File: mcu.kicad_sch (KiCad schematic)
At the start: 15 parts, among them SW1 RST, SW2 BOOT, U1 ESP32-S3-WROOM-1

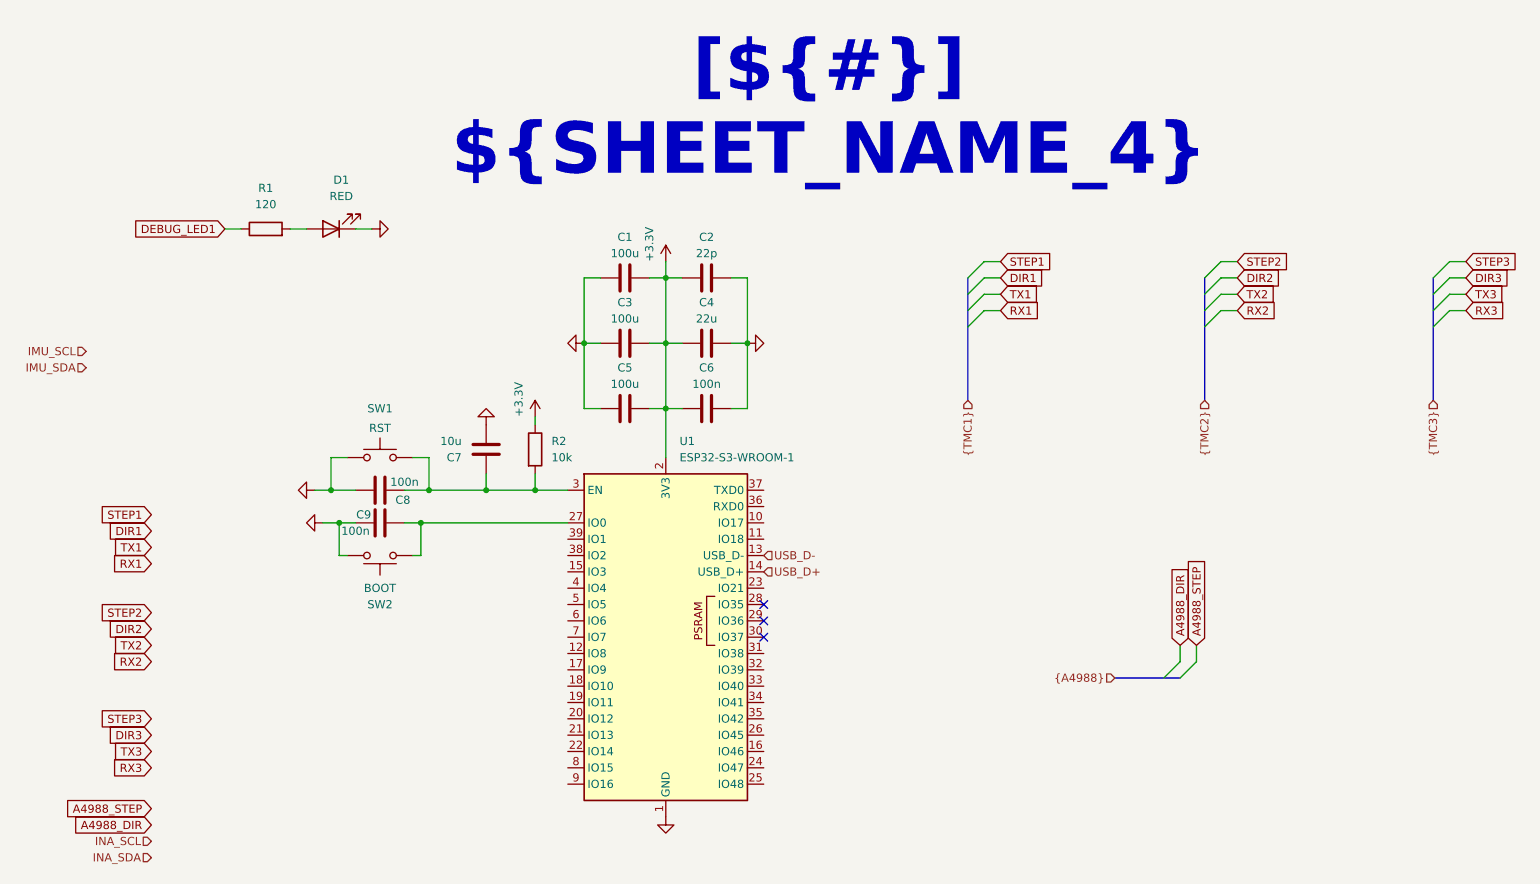
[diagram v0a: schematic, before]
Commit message: Finished design
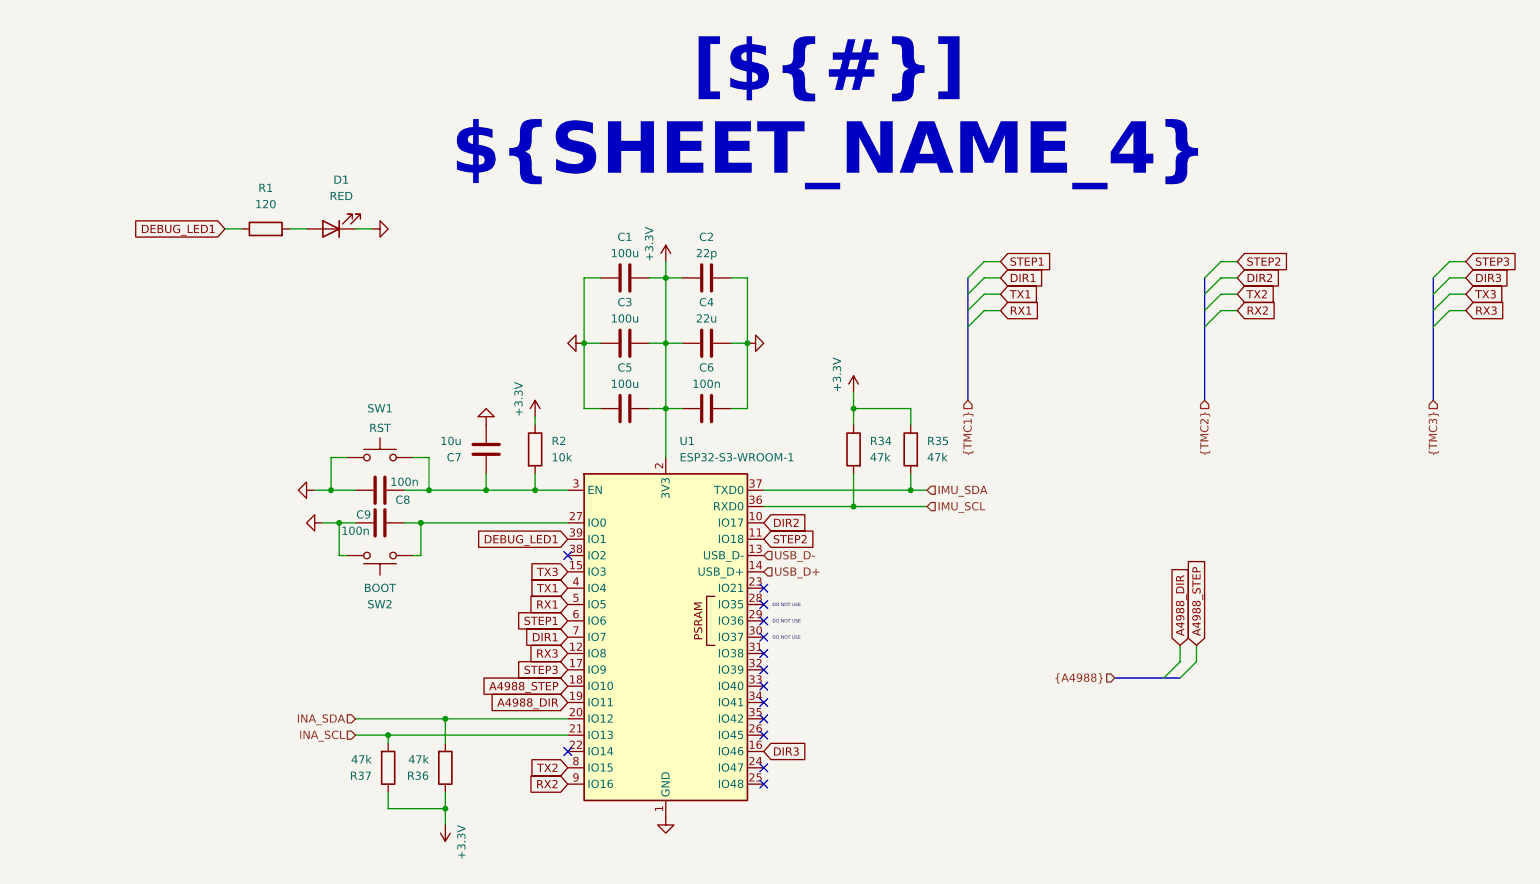
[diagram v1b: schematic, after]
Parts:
- added R34, R35, R36, R37: 47k, Resistor_SMD:R_0603_1608Metric_Pad0.98x0.95mm_HandSolder, symbol Device:R
- C1, C2, C3, C4, C5, C6, C7, C8, C9: footprint (none) -> Capacitor_SMD:C_0603_1608Metric_Pad1.08x0.95mm_HandSolder
- D1: footprint (none) -> LED_SMD:LED_0603_1608Metric_Pad1.05x0.95mm_HandSolder
- R1, R2: footprint (none) -> Resistor_SMD:R_0603_1608Metric_Pad0.98x0.95mm_HandSolder
- U1: footprint (none) -> Project_Components:ESP32-S3-WROOM-1_novias
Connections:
- net +3.3V: now also R34.1, R35.1, R36.1, R37.1
- net A4988_DIR: now also U1.19 (IO11)
- net A4988_STEP: now also U1.18 (IO10)
- net DEBUG_LED1: now also U1.39 (IO1)
- net DIR1: now also U1.7 (IO7)
- net DIR2: now also U1.10 (IO17)
- net DIR3: now also U1.16 (IO46)
- net IMU_SCL: now also U1.36 (RXD0), R34.2
- net IMU_SDA: now also U1.37 (TXD0), R35.2
- net INA_SCL: now also U1.21 (IO13), R37.2
- net INA_SDA: now also U1.20 (IO12), R36.2
- net RX1: now also U1.5 (IO5)
- net RX2: now also U1.9 (IO16)
- net RX3: now also U1.12 (IO8)
- net STEP1: now also U1.6 (IO6)
- net STEP2: now also U1.11 (IO18)
- net STEP3: now also U1.17 (IO9)
- net TX1: now also U1.4 (IO4)
- net TX2: now also U1.8 (IO15)
- net TX3: now also U1.15 (IO3)
- no-connect marks 3 -> 14
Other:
- note added: "DO NOT USE"

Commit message: Final tweaks
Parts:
- C1, C3, C5: footprint Capacitor_SMD:C_0603_1608Metric_Pad1.08x0.95mm_HandSolder -> Capacitor_SMD:C_1206_3216Metric_Pad1.33x1.80mm_HandSolder
- SW1, SW2: footprint Button_Switch_SMD:Panasonic_EVQPUJ_EVQPUA -> Button_Switch_SMD:SW_SPST_PTS647_Sx38
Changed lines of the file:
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@@
 			)
 		)
-		(property "Footprint" "Capacitor_SMD:C_0603_1608Metric_Pad1.08x0.95mm_HandSolder"
+		(property "Footprint" "Capacitor_SMD:C_1206_3216Metric_Pad1.33x1.80mm_HandSolder"
 			(at 118.11 53.6448 0)
 			(hide yes)
@@
 			)
 		)
-		(property "Footprint" "Button_Switch_SMD:Panasonic_EVQPUJ_EVQPUA"
+		(property "Footprint" "Button_Switch_SMD:SW_SPST_PTS647_Sx38"
 			(at 76.2 102.87 0)
 			(hide yes)
@@
 			)
 		)
-		(property "Footprint" "Capacitor_SMD:C_0603_1608Metric_Pad1.08x0.95mm_HandSolder"
+		(property "Footprint" "Capacitor_SMD:C_1206_3216Metric_Pad1.33x1.80mm_HandSolder"
 			(at 118.11 63.8048 0)
 			(hide yes)
@@
 			)
 		)
-		(property "Footprint" "Button_Switch_SMD:Panasonic_EVQPUJ_EVQPUA"
+		(property "Footprint" "Button_Switch_SMD:SW_SPST_PTS647_Sx38"
 			(at 76.2 77.47 0)
 			(hide yes)
@@
 			)
 		)
-		(property "Footprint" "Capacitor_SMD:C_0603_1608Metric_Pad1.08x0.95mm_HandSolder"
+		(property "Footprint" "Capacitor_SMD:C_1206_3216Metric_Pad1.33x1.80mm_HandSolder"
 			(at 118.11 73.9648 0)
 			(hide yes)
